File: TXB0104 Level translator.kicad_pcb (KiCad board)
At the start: 2 copper layers, 5 parts, among them P1 CONN_7, P2 CONN_7, U1 TXB0104

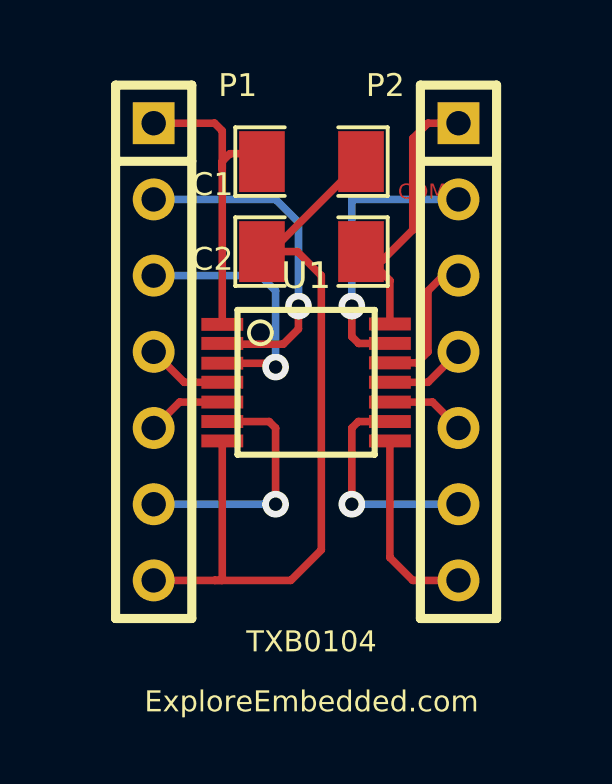
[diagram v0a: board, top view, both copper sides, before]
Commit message: Ready for manufacturing
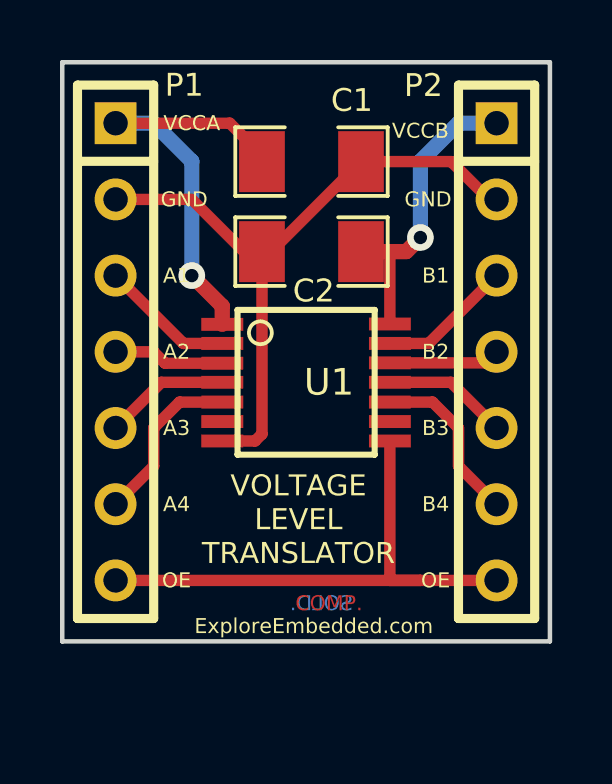
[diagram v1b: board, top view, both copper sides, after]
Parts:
- moved P1 1.27 mm to (77.5, 53.3)
- moved P2 1.27 mm to (90.2, 53.3)
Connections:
- net N-0000014 renamed +3.3VP
- net N-000009 renamed +5V
- P1 pad 2: N-0000013 -> GND
- P1 pad 3: N-0000012 -> Net-(P1-Pad3)
- P1 pad 4: N-0000011 -> Net-(P1-Pad4)
- P1 pad 5: N-000007 -> Net-(P1-Pad5)
- P1 pad 6: N-0000010 -> Net-(P1-Pad6)
- P1 pad 7: GND -> /OE
- P2 pad 2: N-000006 -> GND
- P2 pad 3: N-000005 -> Net-(P2-Pad3)
- P2 pad 4: N-000001 -> Net-(P2-Pad4)
- P2 pad 5: N-000004 -> Net-(P2-Pad5)
- P2 pad 6: N-000003 -> Net-(P2-Pad6)
- P2 pad 7: N-000002 -> /OE
- U1 pad 10: N-000004 -> Net-(P2-Pad6)
- U1 pad 11: N-000001 -> Net-(P2-Pad5)
- U1 pad 12: N-000005 -> Net-(P2-Pad4)
- U1 pad 13: N-000006 -> Net-(P2-Pad3)
- U1 pad 2: N-0000013 -> Net-(P1-Pad3)
- U1 pad 3: N-0000012 -> Net-(P1-Pad4)
- U1 pad 4: N-0000011 -> Net-(P1-Pad5)
- U1 pad 5: N-000007 -> Net-(P1-Pad6)
- U1 pad 6: N-0000010 -> Net-(U1-Pad6)
- U1 pad 8: N-000002 -> /OE
- U1 pad 9: N-000003 -> Net-(U1-Pad9)
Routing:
- net /OE: track 0.00 -> 18.4 mm
- net N-0000013: track 11.5 -> 0.00 mm, vias 1 -> 0
- net N-000006: track 9.49 -> 0.00 mm, vias 1 -> 0
- net N-0000012: track 8.65 -> 0.00 mm, vias 1 -> 0
- net N-0000010: track 8.47 -> 0.00 mm, vias 1 -> 0
- net N-000003: track 7.46 -> 0.00 mm, vias 1 -> 0
- net N-000002: track 6.49 -> 0.00 mm
- net Net-(P2-Pad6): track 0.00 -> 5.71 mm
- net Net-(P1-Pad6): track 0.00 -> 5.71 mm
- net N-000005: track 4.68 -> 0.00 mm
- net Net-(P2-Pad3): track 0.00 -> 4.49 mm
- net Net-(P1-Pad3): track 0.00 -> 4.49 mm
- net GND: track 26.9 -> 22.4 mm
- net Net-(P2-Pad5): track 0.00 -> 4.19 mm
- net Net-(P1-Pad5): track 0.00 -> 4.19 mm
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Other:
- board outline added: 16.3 x 19.3 mm
- net class Default: trace_width 0.254 -> 0.15
- rule trace_min: 0.254 -> 0.15
- board text added: "A1"
- board text added: "A2"
- board text added: "A3"
- board text added: "A4"
- board text added: "B1"
- board text added: "B2"
- board text added: "B3"
- board text added: "B4"
- board text added: "GND"
- board text added: "OE"
- board text added: "SOLD."
- board text added: "VCCA"
- board text added: "VCCB"
- board text added: "VOLTAGE LEVEL TRANSLATOR"
- board text removed: "TXB0104"
